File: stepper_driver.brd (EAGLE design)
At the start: 100 x 80 mm, 12 parts, among them IC1 L293D, IC2 L293D, Q1 IRLML5203, Q2 IRLML5203

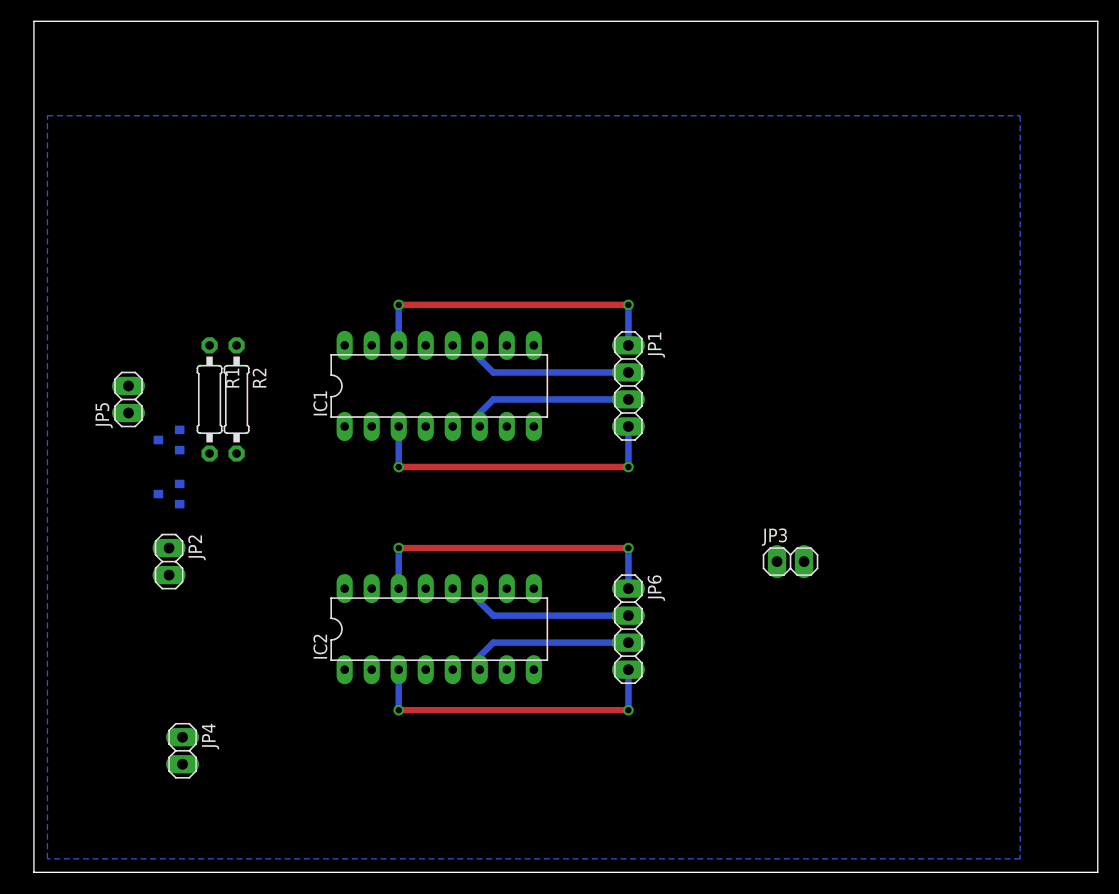
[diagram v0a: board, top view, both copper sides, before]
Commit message: First draft artwork done
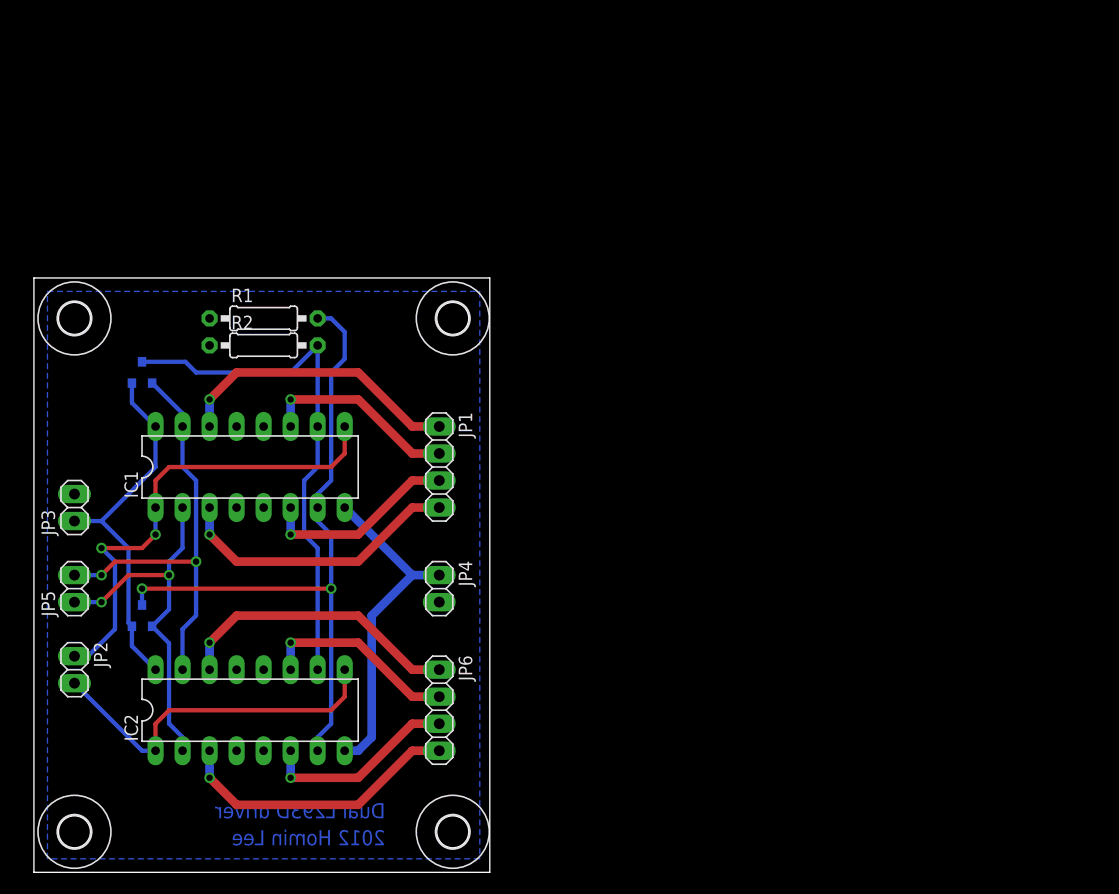
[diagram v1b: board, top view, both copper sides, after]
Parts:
- added U$6, U$7, U$8, U$9: (no value), holes:3,0
- moved JP3 67.5 mm to (3.81, 34.3), turned to 90 degrees
- moved JP4 28.5 mm to (38.1, 26.7)
- moved IC1 19.3 mm to (20.3, 38.1)
- moved IC2 19.3 mm to (20.3, 15.2)
- moved JP1 19.3 mm to (38.1, 38.1)
- moved JP6 19.3 mm to (38.1, 15.2)
- moved JP5 18.5 mm to (3.81, 26.7)
- moved JP2 13.5 mm to (3.81, 19.1)
- moved Q1 11.7 mm to (10.2, 24.1), turned to 0 degrees
- moved R1 9.16 mm to (21.6, 52.1), turned to 0 degrees
- moved Q2 6.84 mm to (10.2, 47.0), turned to 0 degrees
- moved R2 5.68 mm to (21.6, 49.5), turned to 0 degrees
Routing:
- net N$5: track 0.00 -> 63.9 mm, vias 0 -> 2
- net N$7: track 0.00 -> 49.5 mm
- net IC1_EN: track 0.00 -> 45.1 mm, vias 0 -> 2
- net S2: track 0.00 -> 41.1 mm, vias 0 -> 2
- net S1: track 0.00 -> 35.2 mm, vias 0 -> 2
- net 5V: track 0.00 -> 34.6 mm
- net IC2_EN: track 0.00 -> 34.2 mm
- net VCC: track 0.00 -> 31.4 mm
- net N$3: track 15.8 -> 18.6 mm, vias 0 -> 1
- net N$8: track 15.8 -> 18.6 mm, vias 0 -> 1
- net N$9: track 15.8 -> 18.6 mm, vias 0 -> 1
- net N$2: track 15.8 -> 18.6 mm, vias 0 -> 1
- net N$6: track 29.2 -> 27.3 mm, vias 2 -> 1
- net N$11: track 29.2 -> 27.3 mm, vias 2 -> 1
- net N$4: track 29.2 -> 27.3 mm, vias 2 -> 1
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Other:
- board size 100 x 80 mm -> 42.9 x 55.9 mm
- board text added: "2012 Homin Lee"
- board text added: "Dual L293D driver"

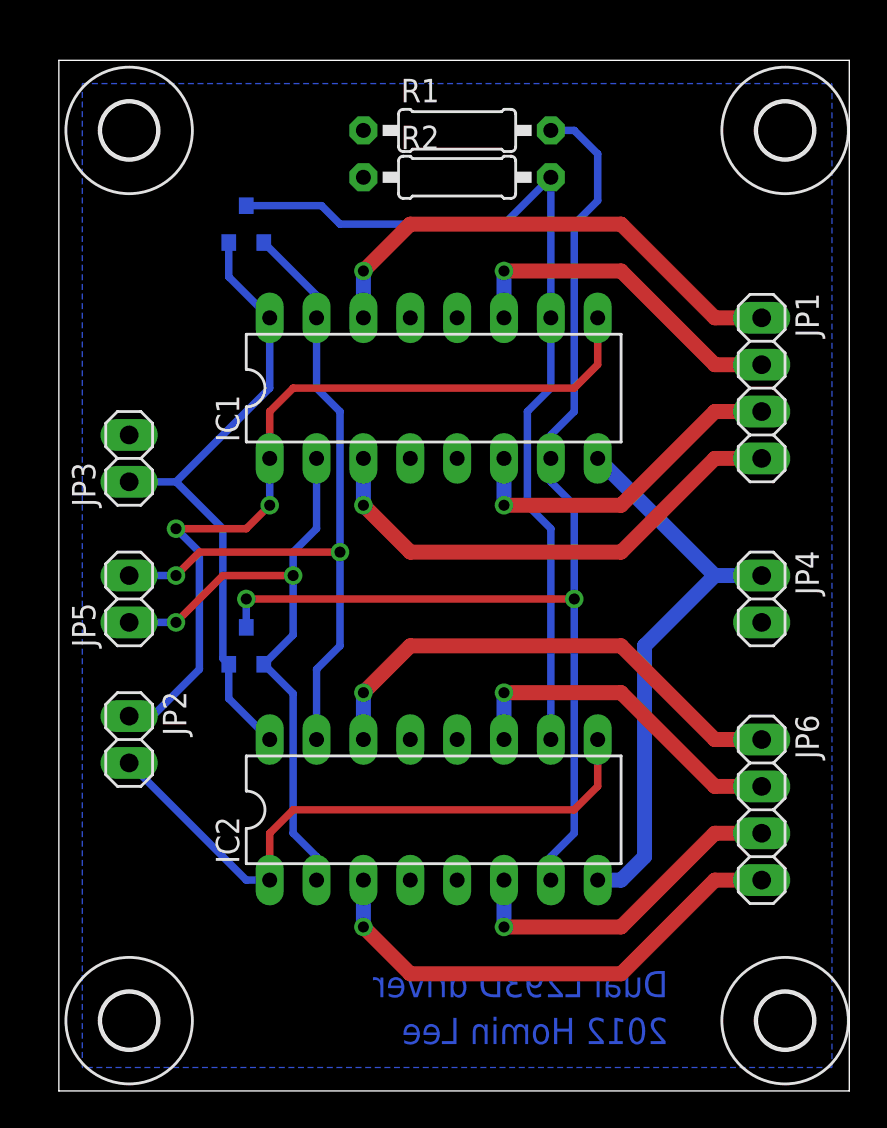
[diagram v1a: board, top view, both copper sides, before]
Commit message: Polishing artwork
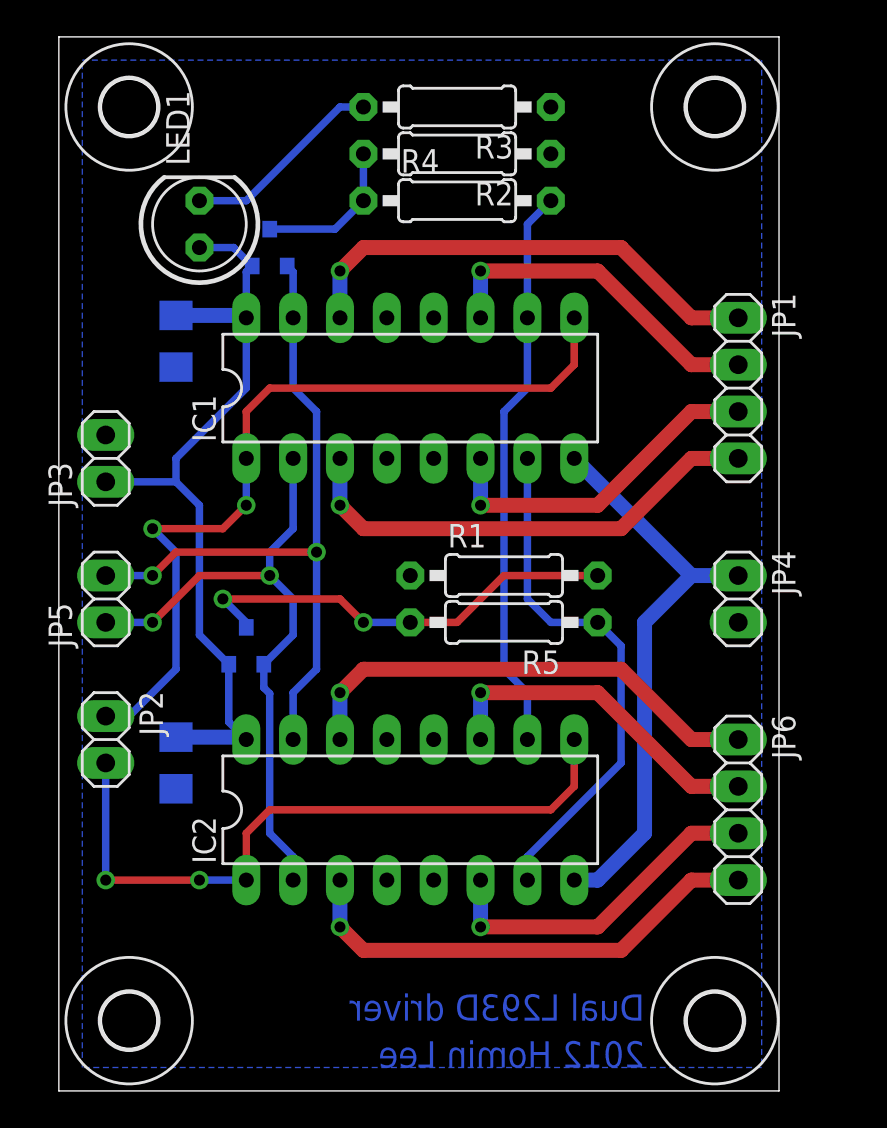
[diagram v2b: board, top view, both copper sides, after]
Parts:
- added C1, C2: (no value), rcl:C1206
- added LED1: (no value), led:LED5MM
- added R3, R4, R5: 1k, rcl:0207/10
- R1, R2: value (none) -> 10k
- moved R1 24.3 mm to (24.1, 27.9)
- moved U$7 4.02 mm to (35.6, 53.3)
- moved U$9 3.81 mm to (35.6, 3.81)
- moved Q2 1.80 mm to (11.4, 45.7)
- moved JP1 1.27 mm to (36.8, 38.1)
- moved JP4 1.27 mm to (36.8, 26.7)
- moved JP6 1.27 mm to (36.8, 15.2)
- moved U$8 1.27 mm to (3.81, 53.3)
- moved JP2 1.27 mm to (2.54, 19.1)
- moved JP3 1.27 mm to (2.54, 34.3)
- moved JP5 1.27 mm to (2.54, 26.7)
- moved IC1 1.27 mm to (19.1, 38.1)
- moved IC2 1.27 mm to (19.1, 15.2)
- moved R2 1.27 mm to (21.6, 50.8), turned to 180 degrees
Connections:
- new net N$10: LED1.K, R3.2
- new net N$12: Q1.3, R1.2, R5.2
- new net N$13: Q2.3, R2.2, R4.1
- net 5V: now also C1.1, C2.1, LED1.A
- net GND: now also C1.2, C2.2, R3.1
- net N$5: now also R5.1; no longer Q1.3, R1.2
- net N$7: now also R4.2; no longer Q2.3, R2.2
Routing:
- net N$5: track 63.9 -> 28.6 mm, vias 2 -> 0
- net N$12: track 0.00 -> 24.0 mm, vias 0 -> 2
- net N$7: track 49.5 -> 30.8 mm
- net N$10: track 0.00 -> 11.0 mm
- net 5V: track 34.6 -> 43.8 mm
- net N$13: track 0.00 -> 8.26 mm
- net IC2_EN: track 34.2 -> 37.9 mm, vias 0 -> 2
- net S2: track 41.1 -> 38.8 mm
- net N$6: track 27.3 -> 26.2 mm
- net N$4: track 27.3 -> 26.2 mm
- net N$11: track 27.3 -> 26.2 mm
- net N$1: track 27.3 -> 26.2 mm
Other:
- board size 42.9 x 55.9 mm -> 39 x 57.1 mm
